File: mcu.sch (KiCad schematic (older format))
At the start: 17 parts, among them U201 STM32F072C8Tx, Y201 8MHz

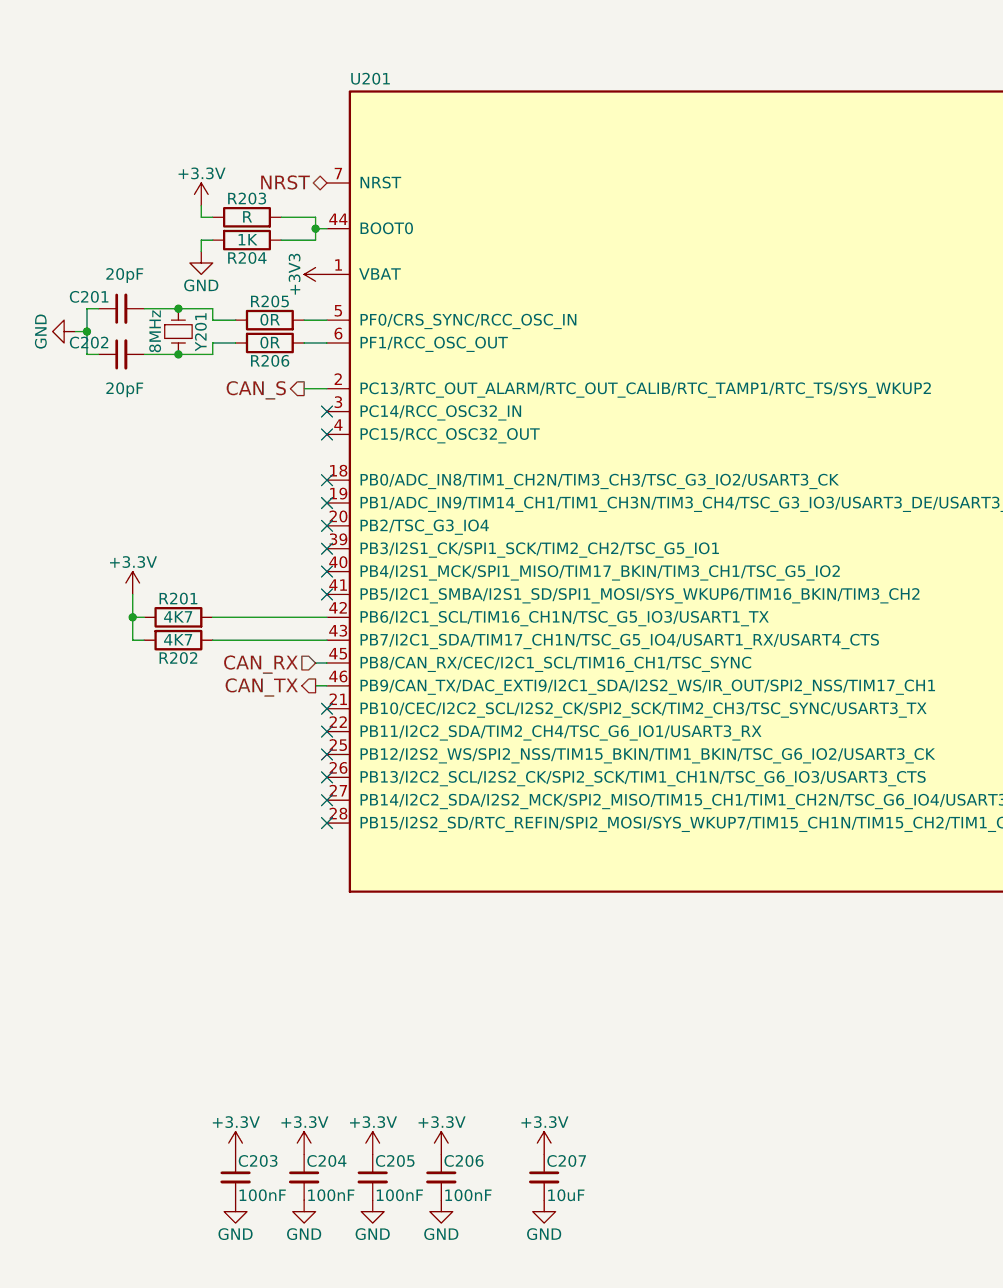
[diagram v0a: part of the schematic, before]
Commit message: add testpoints, reset line cap
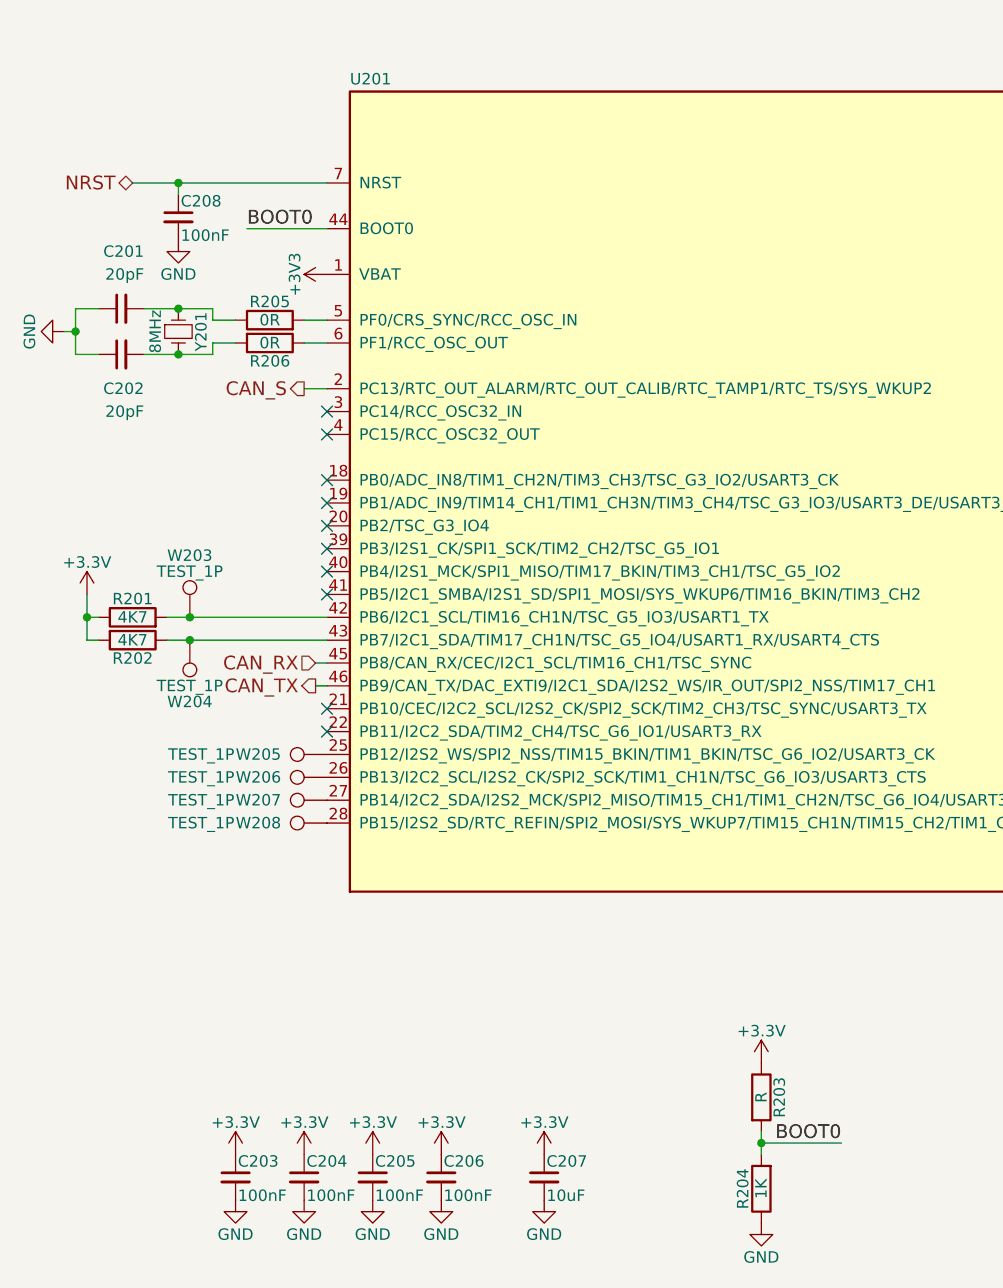
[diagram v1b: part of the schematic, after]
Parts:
- added C208: 100nF, Capacitors_SMD:C_0603, symbol C_Small
- added W203, W204, W205, W206, W207, W208: TEST_1P, Measurement_Points:Measurement_Point_Round-SMD-Pad_Small, symbol TEST_1P
- R203: footprint Resistors_SMD:R_0603 -> Resistors_SMD:R_0805
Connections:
- net GND: now also R204.1, C208.2; no longer R204.2
- net NRST: now also C208.1
- net at U201.25 (PB12/I2S2_WS/SPI2_NSS/TIM15_BKIN/TIM1_BKIN/TSC_G6_IO2/USART3_CK): now also W205.1
- net at U201.26 (PB13/I2C2_SCL/I2S2_CK/SPI2_SCK/TIM1_CH1N/TSC_G6_IO3/USART3_CTS): now also W206.1
- net at U201.27 (PB14/I2C2_SDA/I2S2_MCK/SPI2_MISO/TIM15_CH1/TIM1_CH2N/TSC_G6_IO4/USART3_DE/USART3_RTS): now also W207.1
- net at U201.28 (PB15/I2S2_SD/RTC_REFIN/SPI2_MOSI/SYS_WKUP7/TIM15_CH1N/TIM15_CH2/TIM1_CH3N): now also W208.1
- net at R201.2, U201.42 (PB6/I2C1_SCL/TIM16_CH1N/TSC_G5_IO3/USART1_TX): now also W203.1
- net at R202.1, U201.43 (PB7/I2C1_SDA/TIM17_CH1N/TSC_G5_IO4/USART1_RX/USART4_CTS): now also W204.1
- net BOOT0: now reaches R203.2, U201.44 (BOOT0)
- net BOOT0: now also R204.2; no longer R204.1
- no-connect marks 22 -> 18
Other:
- moved on the sheet: R201, R202, R203, R204
